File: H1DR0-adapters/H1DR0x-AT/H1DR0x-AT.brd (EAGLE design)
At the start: 34.6 x 30 mm, 3 parts, among them X1 CON-PHOENIX-350_1751277

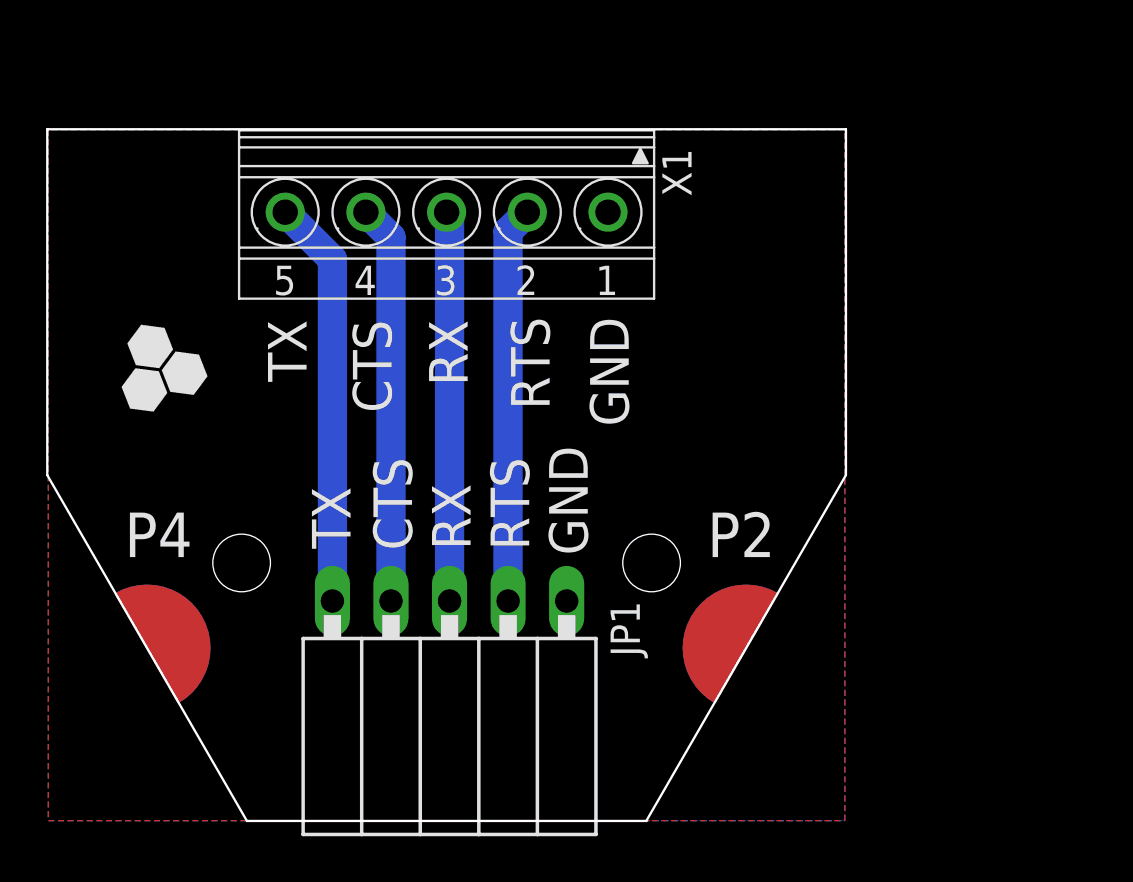
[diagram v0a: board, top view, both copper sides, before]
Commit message: no message
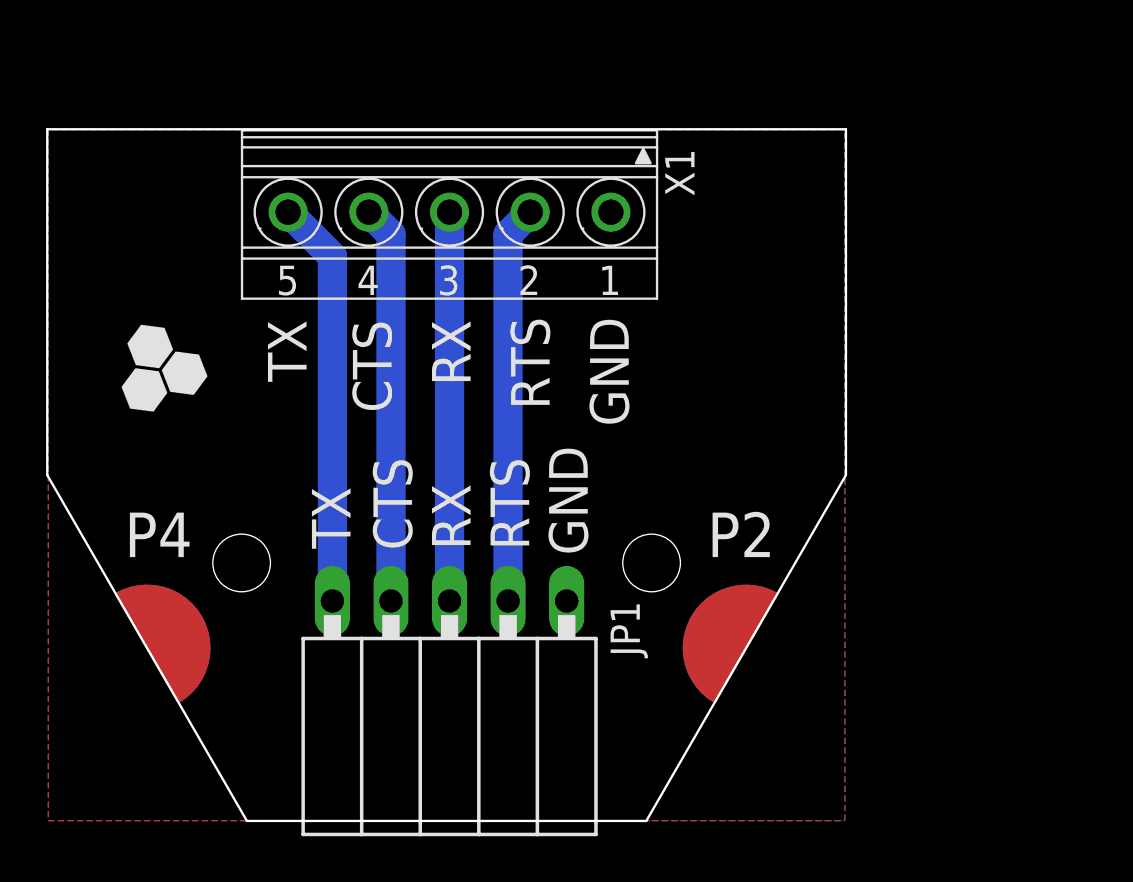
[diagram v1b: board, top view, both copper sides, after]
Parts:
- moved X1 0.13 mm to (7.11, 22.9)
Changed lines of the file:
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@@
 <text x="13.208" y="18.415" size="1.6764" layer="21" rot="R270">GND</text>
 <text x="9.779" y="18.415" size="1.6764" layer="21" rot="R270">RTS</text>
-<text x="6.223" y="18.288" size="1.6764" layer="21" rot="R270">RX</text>
+<text x="6.35" y="18.288" size="1.6764" layer="21" rot="R270">RX</text>
 <text x="2.921" y="18.288" size="1.6764" layer="21" rot="R270">CTS</text>
 <text x="14.351" y="16.764" size="1.9304" layer="22" rot="MR0">H1DR0x-AT</text>
@@
 </autorouter>
 <elements>
-<element name="X1" library="Hexabitz" package="CON-PHOENIX-350_1751277" value="CON-PHOENIX-350_1751277" x="6.985" y="22.86" smashed="yes" rot="R180">
-<attribute name="MF" value="" x="6.985" y="22.86" size="1.778" layer="27" rot="R180" display="off"/>
-<attribute name="MPN" value="" x="6.985" y="22.86" size="1.778" layer="27" rot="R180" display="off"/>
-<attribute name="NAME" x="16.34" y="25.7175" size="1.27" layer="25" rot="R270"/>
-<attribute name="OC_FARNELL" value="unknown" x="6.985" y="22.86" size="1.778" layer="27" rot="R180" display="off"/>
-<attribute name="OC_NEWARK" value="unknown" x="6.985" y="22.86" size="1.778" layer="27" rot="R180" display="off"/>
+<element name="X1" library="Hexabitz" package="CON-PHOENIX-350_1751277" value="CON-PHOENIX-350_1751277" x="7.112" y="22.86" smashed="yes" rot="R180">
+<attribute name="MF" value="" x="7.112" y="22.86" size="1.778" layer="27" rot="R180" display="off"/>
+<attribute name="MPN" value="" x="7.112" y="22.86" size="1.778" layer="27" rot="R180" display="off"/>
+<attribute name="NAME" x="16.467" y="25.7175" size="1.27" layer="25" rot="R270"/>
+<attribute name="OC_FARNELL" value="unknown" x="7.112" y="22.86" size="1.778" layer="27" rot="R180" display="off"/>
+<attribute name="OC_NEWARK" value="unknown" x="7.112" y="22.86" size="1.778" layer="27" rot="R180" display="off"/>
 </element>
 <element name="JP1" library="Hexabitz" package="F_1X05" value="" x="7.112" y="3.556" smashed="yes" rot="R180">
@@
 <contactref element="X1" pad="3"/>
 <contactref element="JP1" pad="3"/>
-<wire x1="7.112" y1="6.096" x2="7.112" y2="22.833" width="1.27" layer="16"/>
-<wire x1="7.112" y1="22.833" x2="6.985" y2="22.96" width="1.27" layer="16"/>
+<wire x1="7.112" y1="6.096" x2="7.112" y2="22.96" width="1.27" layer="16"/>
 </signal>
 <signal name="RTS_OUT">
 <contactref element="X1" pad="2"/>
-<wire x1="9.652" y1="22.127" x2="10.485" y2="22.96" width="1.27" layer="16"/>
+<wire x1="9.652" y1="22" x2="10.612" y2="22.96" width="1.27" layer="16"/>
 <contactref element="JP1" pad="2"/>
-<wire x1="9.652" y1="6.096" x2="9.652" y2="22.127" width="1.27" layer="16"/>
+<wire x1="9.652" y1="6.096" x2="9.652" y2="22" width="1.27" layer="16"/>
 </signal>
 <signal name="TX_OUT">
 <contactref element="X1" pad="5"/>
 <contactref element="JP1" pad="5"/>
-<wire x1="2.032" y1="20.913" x2="2.032" y2="6.096" width="1.27" layer="16"/>
-<wire x1="-0.015" y1="22.96" x2="2.032" y2="20.913" width="1.27" layer="16"/>
+<wire x1="2.032" y1="21.04" x2="2.032" y2="6.096" width="1.27" layer="16"/>
+<wire x1="0.112" y1="22.96" x2="2.032" y2="21.04" width="1.27" layer="16"/>
 </signal>
 <signal name="CTS_OUT">
 <contactref element="X1" pad="4"/>
 <contactref element="JP1" pad="4"/>
-<wire x1="4.572" y1="6.096" x2="4.572" y2="21.873" width="1.27" layer="16"/>
-<wire x1="4.572" y1="21.873" x2="3.485" y2="22.96" width="1.27" layer="16"/>
+<wire x1="4.572" y1="6.096" x2="4.572" y2="22" width="1.27" layer="16"/>
+<wire x1="4.572" y1="22" x2="3.612" y2="22.96" width="1.27" layer="16"/>
 </signal>
 </signals>

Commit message: no message
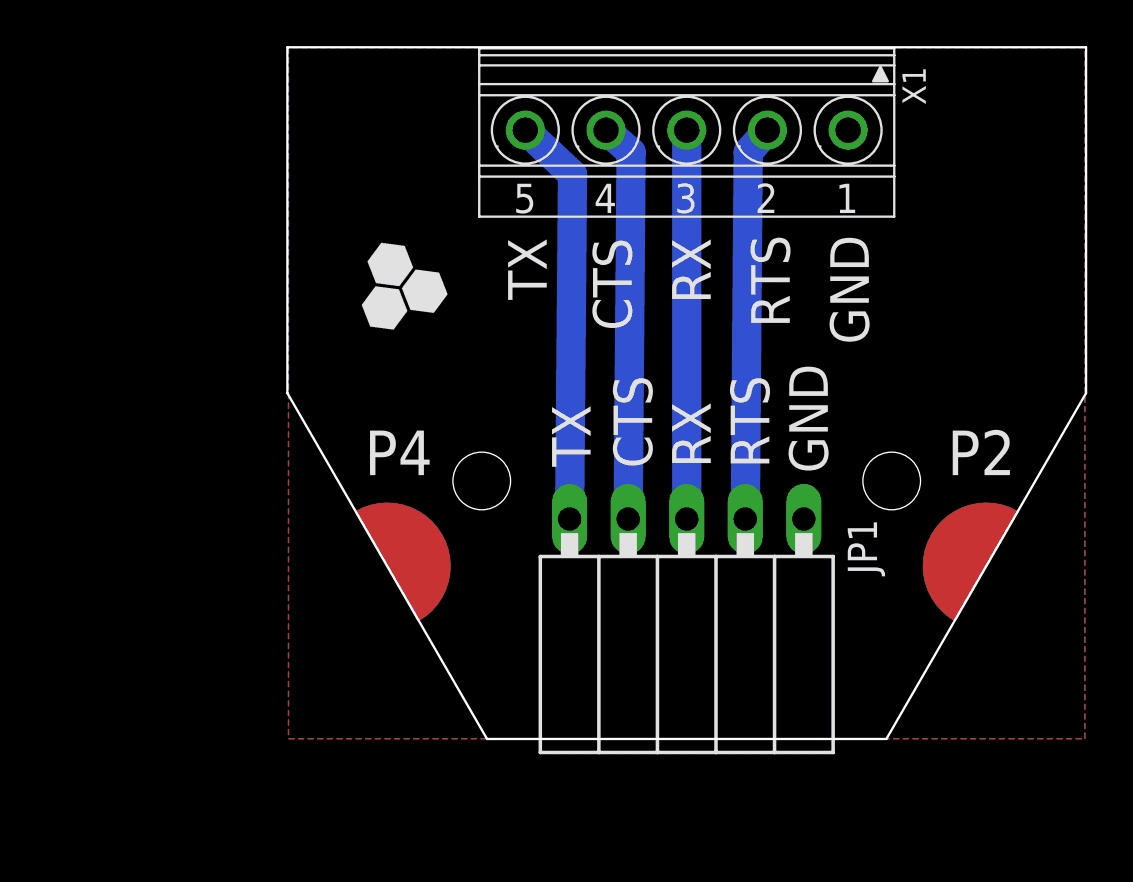
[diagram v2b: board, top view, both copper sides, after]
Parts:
- moved U$1 11.0 mm to (17.4, 15.1)
- moved JP1 10.9 mm to (17.4, 7.11)
- moved X1 10.9 mm to (17.4, 26.4)
